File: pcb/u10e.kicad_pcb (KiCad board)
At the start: 2 copper layers, 151 x 117 mm, 57 parts, among them J1 MJ-4PP-9, K11 KEYSW, K12 KEYSW, K13 KEYSW, K14 KEYSW, K15 KEYSW, K16 KEYSW, K21 KEYSW, K22 KEYSW, K23 KEYSW, K24 KEYSW, K25 KEYSW, K26 KEYSW, K31 KEYSW, K32 KEYSW, K33 KEYSW, K34 KEYSW, K35 KEYSW, K36 KEYSW, K41 KEYSW, K42 KEYSW, K43 KEYSW, K44 KEYSW, K45 KEYSW, K46 KEYSW, K51 KEYSW, K52 KEYSW, K53 KEYSW, SW1 SW_PUSH_RESET, U1 ProMicro

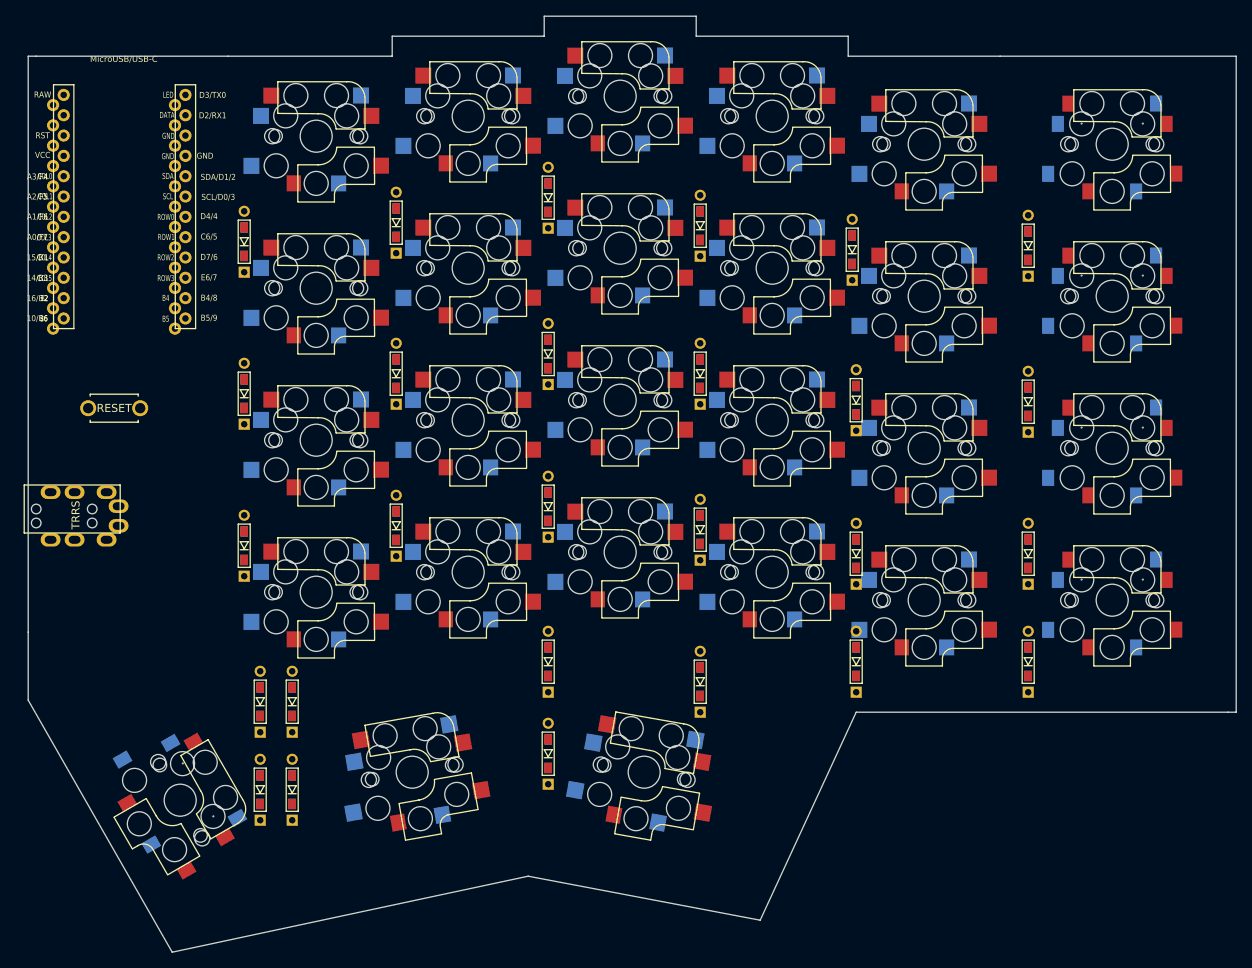
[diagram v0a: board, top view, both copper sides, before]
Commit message: pre routing commit
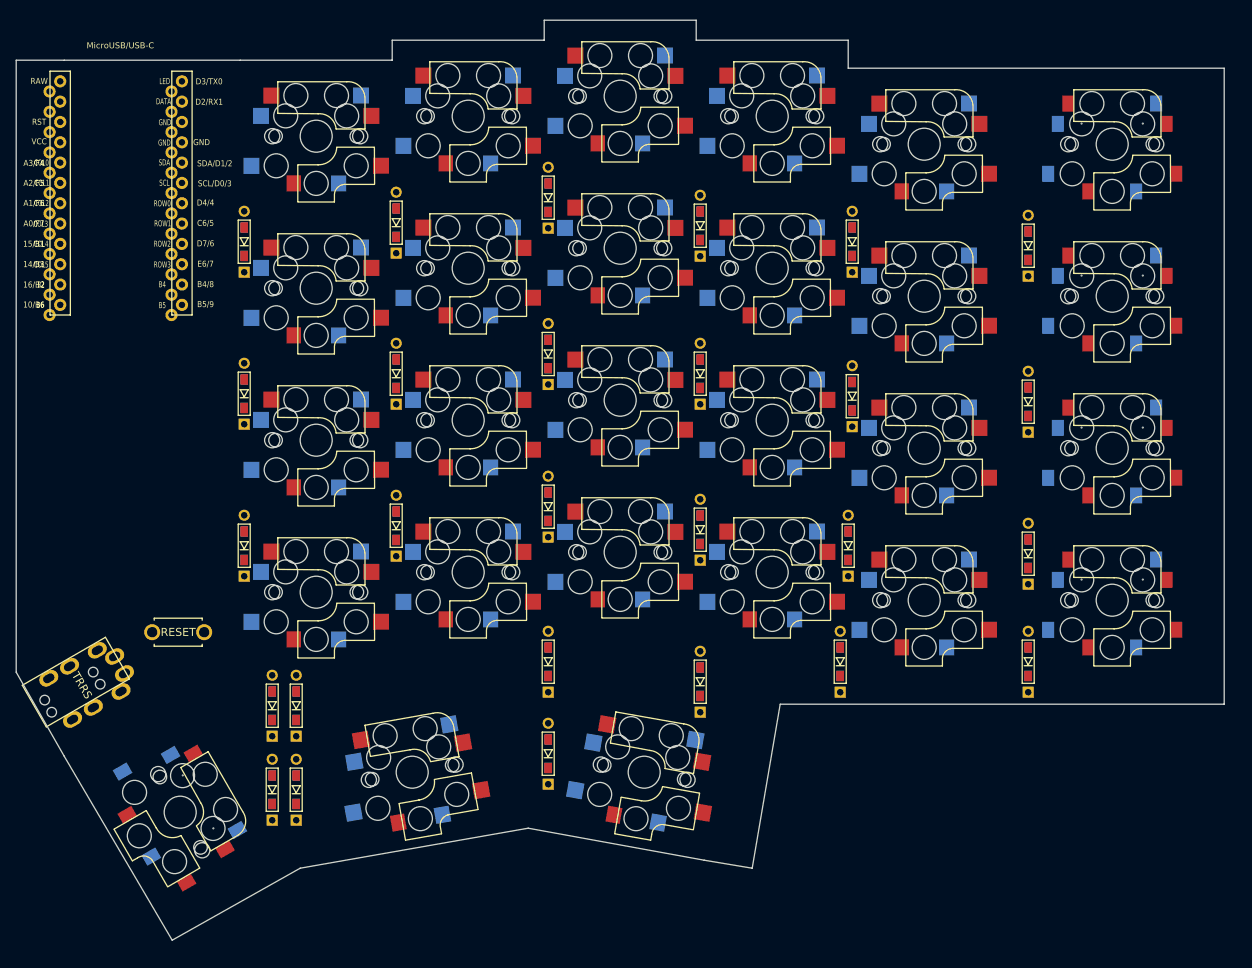
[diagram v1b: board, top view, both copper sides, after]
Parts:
- moved SW1 29.1 mm to (47.8, 90.0)
- moved J1 24.7 mm to (29.8, 99.2), turned to 120 degrees
- moved D45 2.00 mm to (130.5, 93.7)
- moved U1 1.76 mm to (40.6, 35.6)
- moved D41 1.58 mm to (59.5, 99.2)
- moved D51 1.50 mm to (59.5, 109.7)
- moved K51 1.50 mm to (48.0, 112.5)
- moved D35 1.41 mm to (131.5, 79.2)
- moved D15 1.00 mm to (132.0, 41.2)
- moved D25 0.71 mm to (132.0, 60.5)
- moved D42 0.71 mm to (62.5, 99.2)
- moved D52 0.50 mm to (62.5, 109.7)
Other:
- board size 151 x 117 mm -> 151 x 115 mm
